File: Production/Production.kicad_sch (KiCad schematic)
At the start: 28 parts, among them IC1 MAX3323EEPE+, J1 530480510, J2 530480410, J3 USB4085-GF-A_REVB, U1 BD33FC0FP-E2, U2 ADR02AUJZ-REEL7, U3 ATSAMD21G18A-AUT, Y1 32.768, 12.5pF

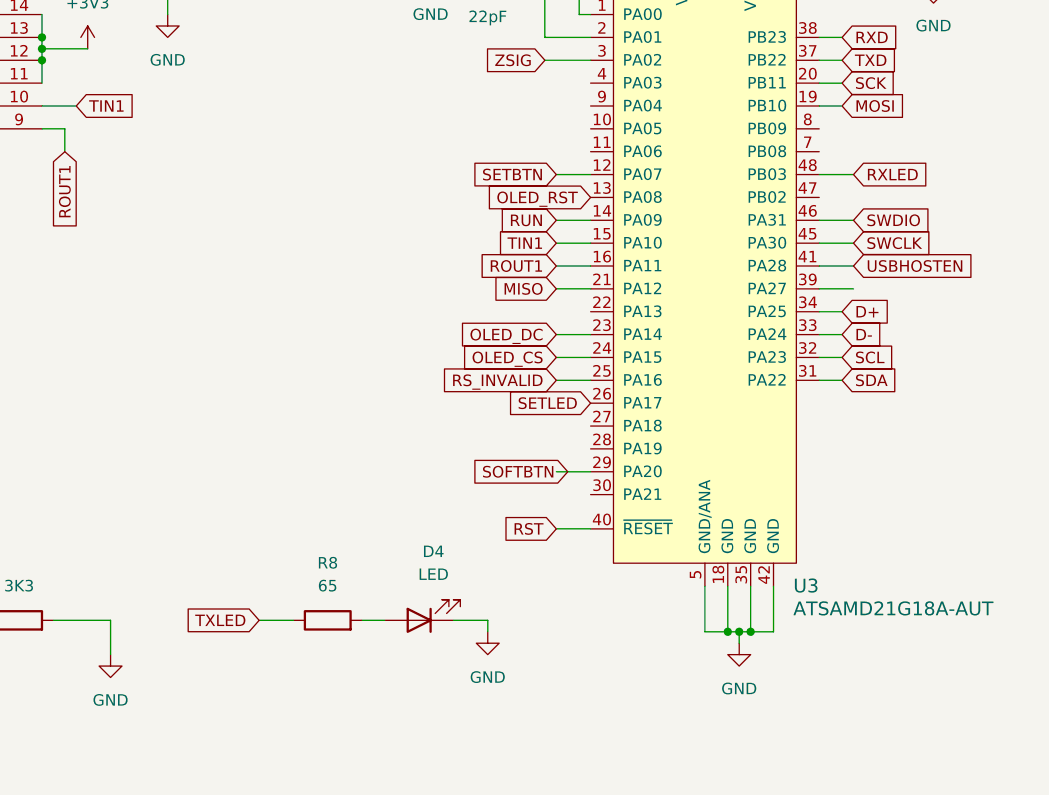
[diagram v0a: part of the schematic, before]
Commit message: I layout
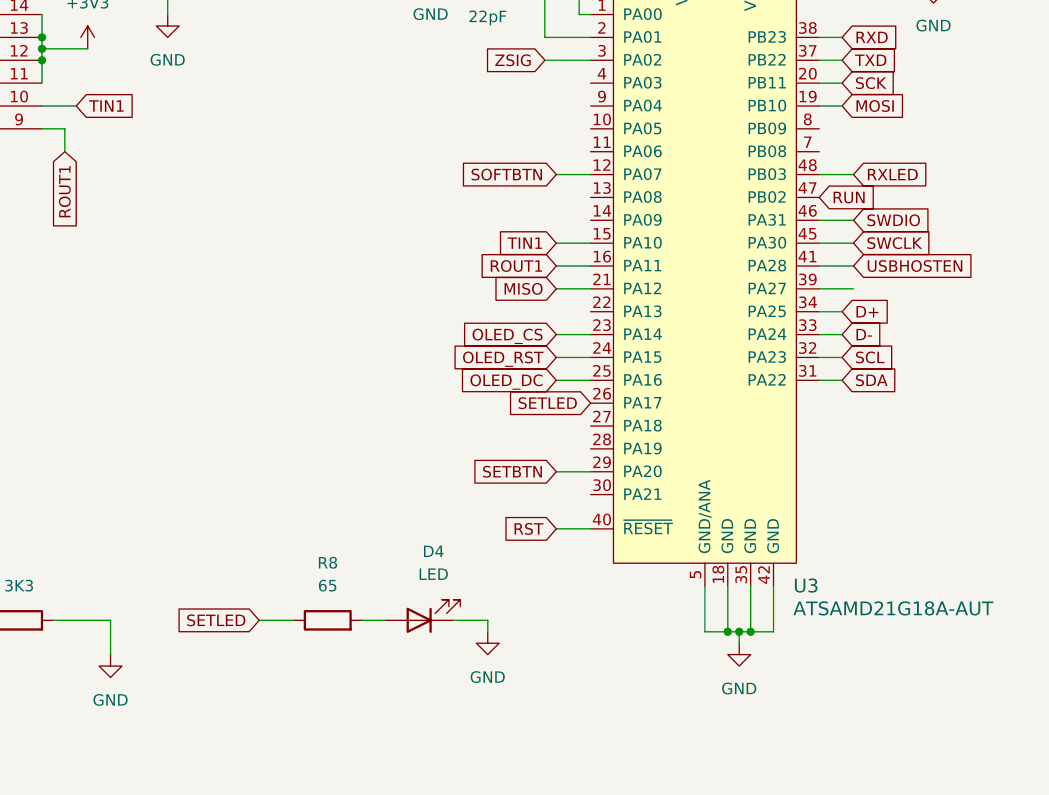
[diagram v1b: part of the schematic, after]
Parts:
- C1, C13, C2, C3, C4, C5, C6, C7, C8: footprint Capacitor_SMD:C_0805_2012Metric -> Capacitor_SMD:C_0504_1310Metric
- J2: footprint Connector_Molex:Molex_PicoBlade_53048-0410_1x04_P1.25mm_Horizontal -> Connector_Molex_2:Molex_PicoBlade_53048-0410_1x04_P1.25mm_Horizontal
- R1, R2, R3, R5, R8: footprint Resistor_SMD:R_0805_2012Metric -> Resistor_SMD:R_0603_1608Metric
- U2: footprint Package_TO_SOT_SMD:TSOT-23-5_HandSoldering -> Package_TO_SOT_SMD:TSOT-23-5
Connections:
- net RS_INVALID is gone; now on net OLED_DC: U3.25 (PA16)
- net TXLED is gone; now on net SETLED: R8.1
- net OLED_CS: now also U3.23 (PA14); no longer U3.24 (PA15)
- net OLED_DC: no longer U3.23 (PA14)
- net OLED_RST: now also U3.24 (PA15); no longer U3.13 (PA08)
- net RUN: now also U3.47 (PB02); no longer U3.14 (PA09)
- net SETBTN: now also U3.29 (PA20); no longer U3.12 (PA07)
- net SOFTBTN: now also U3.12 (PA07); no longer U3.29 (PA20)
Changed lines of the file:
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@@
 	(wire
 		(pts
-			(xy 227.33 99.06) (xy 231.14 99.06)
-		)
-		(stroke
-			(width 0)
-			(type default)
-		)
-	)
-	(wire
-		(pts
 			(xy 105.41 165.1) (xy 107.95 165.1)
 		)
@@
 		)
 	)
-	(global_label "TXLED"
+	(global_label "MOSI"
 		(shape input)
-		(at 194.31 143.51 180)
+		(at 259.08 86.36 0)
 		(fields_autoplaced yes)
 		(effects
@@
 				(size 1.27 1.27)
 			)
-			(justify right)
+			(justify left)
 		)
 		(property "Intersheetrefs" "${INTERSHEET_REFS}"
-			(at 185.7006 143.51 0)
+			(at 266.6614 86.36 0)
 			(effects
 				(font
 					(size 1.27 1.27)
 				)
-				(justify right)
+				(justify left)
 				(hide yes)
 			)
 		)
 	)
-	(global_label "MOSI"
+	(global_label "ZREF"
 		(shape input)
-		(at 259.08 86.36 0)
+		(at 266.7 22.86 90)
 		(fields_autoplaced yes)
 		(effects
@@
 		)
 		(property "Intersheetrefs" "${INTERSHEET_REFS}"
-			(at 266.6614 86.36 0)
+			(at 266.7 15.1577 90)
 			(effects
 				(font
@@
 		)
 	)
-	(global_label "ZREF"
+	(global_label "TXD"
 		(shape input)
-		(at 266.7 22.86 90)
+		(at 259.08 81.28 0)
 		(fields_autoplaced yes)
 		(effects
@@
 		)
 		(property "Intersheetrefs" "${INTERSHEET_REFS}"
-			(at 266.7 15.1577 90)
+			(at 265.5123 81.28 0)
 			(effects
 				(font
@@
 		)
 	)
-	(global_label "TXD"
+	(global_label "SETLED"
 		(shape input)
-		(at 259.08 81.28 0)
+		(at 194.31 143.51 180)
 		(fields_autoplaced yes)
 		(effects
@@
 				(size 1.27 1.27)
 			)
-			(justify left)
+			(justify right)
 		)
 		(property "Intersheetrefs" "${INTERSHEET_REFS}"
-			(at 265.5123 81.28 0)
+			(at 184.5516 143.51 0)
 			(effects
 				(font
 					(size 1.27 1.27)
 				)
-				(justify left)
+				(justify right)
 				(hide yes)
 			)
@@
 	(global_label "OLED_RST"
 		(shape input)
-		(at 231.14 96.52 180)
+		(at 227.33 114.3 180)
 		(fields_autoplaced yes)
 		(effects
@@
 		)
 		(property "Intersheetrefs" "${INTERSHEET_REFS}"
-			(at 218.9625 96.52 0)
+			(at 215.1525 114.3 0)
 			(effects
 				(font
@@
 	(global_label "SOFTBTN"
 		(shape input)
-		(at 228.6 127 180)
+		(at 227.33 93.98 180)
 		(fields_autoplaced yes)
 		(effects
@@
 		)
 		(property "Intersheetrefs" "${INTERSHEET_REFS}"
-			(at 217.4505 127 0)
+			(at 216.1805 93.98 0)
 			(effects
 				(font
@@
 	(global_label "SETBTN"
 		(shape input)
-		(at 227.33 93.98 180)
+		(at 227.33 127 180)
 		(fields_autoplaced yes)
 		(effects
@@
 		)
 		(property "Intersheetrefs" "${INTERSHEET_REFS}"
-			(at 217.4506 93.98 0)
-			(effects
-				(font
-					(size 1.27 1.27)
-				)
-				(justify right)
-				(hide yes)
-			)
-		)
-	)
-	(global_label "RS_INVALID"
-		(shape input)
-		(at 227.33 116.84 180)
-		(fields_autoplaced yes)
-		(effects
-			(font
-				(size 1.27 1.27)
-			)
-			(justify right)
-		)
-		(property "Intersheetrefs" "${INTERSHEET_REFS}"
-			(at 213.8823 116.84 0)
-			(effects
-				(font
-					(size 1.27 1.27)
-				)
-				(justify right)
-				(hide yes)
-			)
-		)
-	)
-	(global_label "RUN"
-		(shape input)
-		(at 227.33 99.06 180)
-		(fields_autoplaced yes)
-		(effects
-			(font
-				(size 1.27 1.27)
-			)
-			(justify right)
-		)
-		(property "Intersheetrefs" "${INTERSHEET_REFS}"
-			(at 220.4138 99.06 0)
+			(at 217.4506 127 0)
 			(effects
 				(font
@@
 		)
 	)
+	(global_label "RUN"
+		(shape input)
+		(at 256.54 96.52 0)
+		(fields_autoplaced yes)
+		(effects
+			(font
+				(size 1.27 1.27)
+			)
+			(justify left)
+		)
+		(property "Intersheetrefs" "${INTERSHEET_REFS}"
+			(at 263.4562 96.52 0)
+			(effects
+				(font
+					(size 1.27 1.27)
+				)
+				(justify left)
+				(hide yes)
+			)
+		)
+	)
 	(global_label "TIN1"
 		(shape input)
@@
 	(global_label "OLED_DC"
 		(shape input)
-		(at 227.33 111.76 180)
+		(at 227.33 116.84 180)
 		(fields_autoplaced yes)
 		(effects
@@
 		)
 		(property "Intersheetrefs" "${INTERSHEET_REFS}"
-			(at 216.0596 111.76 0)
+			(at 216.0596 116.84 0)
 			(effects
 				(font
@@
 	(global_label "OLED_CS"
 		(shape input)
-		(at 227.33 114.3 180)
+		(at 227.33 111.76 180)
 		(fields_autoplaced yes)
 		(effects
@@
 		)
 		(property "Intersheetrefs" "${INTERSHEET_REFS}"
-			(at 216.1201 114.3 0)
+			(at 216.1201 111.76 0)
 			(effects
 				(font
@@
 			)
 		)
-		(property "Footprint" "Capacitor_SMD:C_0805_2012Metric"
+		(property "Footprint" "Capacitor_SMD:C_0504_1310Metric"
 			(at 270.2052 69.85 0)
 			(effects
@@
 			)
 		)
-		(property "Footprint" "Package_TO_SOT_SMD:TSOT-23-5_HandSoldering"
+		(property "Footprint" "Package_TO_SOT_SMD:TSOT-23-5"
 			(at 199.39 27.94 0)
 			(effects
@@
 			)
 		)
-		(property "Footprint" "Capacitor_SMD:C_0805_2012Metric"
+		(property "Footprint" "Capacitor_SMD:C_0504_1310Metric"
 			(at 108.9152 90.17 0)
 			(effects
@@
 			)
 		)
-		(property "Footprint" "Capacitor_SMD:C_0805_2012Metric"
+		(property "Footprint" "Capacitor_SMD:C_0504_1310Metric"
 			(at 118.4148 38.1 0)
 			(effects
@@
 			)
 		)
-		(property "Footprint" "Resistor_SMD:R_0805_2012Metric"
+		(property "Footprint" "Resistor_SMD:R_0603_1608Metric"
 			(at 104.14 156.718 90)
 			(effects
@@
 			)
 		)
-		(property "Footprint" "Capacitor_SMD:C_0805_2012Metric"
+		(property "Footprint" "Capacitor_SMD:C_0504_1310Metric"
 			(at 174.2948 34.29 0)
 			(effects
@@
 			)
 		)
-		(property "Footprint" "Resistor_SMD:R_0805_2012Metric"
+		(property "Footprint" "Resistor_SMD:R_0603_1608Metric"
 			(at 104.14 154.178 90)
 			(effects
@@
 			)
 		)
-		(property "Footprint" "Resistor_SMD:R_0805_2012Metric"
+		(property "Footprint" "Resistor_SMD:R_0603_1608Metric"
 			(at 201.93 145.288 90)
 			(effects
@@
 			)
 		)
-		(property "Footprint" "Capacitor_SMD:C_0805_2012Metric"
+		(property "Footprint" "Capacitor_SMD:C_0504_1310Metric"
 			(at 121.6152 105.41 0)
 			(effects
@@
 			)
 		)
-		(property "Footprint" "Capacitor_SMD:C_0805_2012Metric"
+		(property "Footprint" "Capacitor_SMD:C_0504_1310Metric"
 			(at 108.9152 77.47 0)
 			(effects
@@
 			)
 		)
-		(property "Footprint" "Resistor_SMD:R_0805_2012Metric"
+		(property "Footprint" "Resistor_SMD:R_0603_1608Metric"
 			(at 151.13 145.288 90)
 			(effects
@@
 			)
 		)
-		(property "Footprint" "Resistor_SMD:R_0805_2012Metric"
+		(property "Footprint" "Resistor_SMD:R_0603_1608Metric"
 			(at 167.64 145.288 90)
 			(effects
@@
 			)
 		)
-		(property "Footprint" "Capacitor_SMD:C_0805_2012Metric"
+		(property "Footprint" "Capacitor_SMD:C_0504_1310Metric"
 			(at 223.52 63.8048 0)
 			(effects
@@
 			)
 		)
-		(property "Footprint" "Capacitor_SMD:C_0805_2012Metric"
+		(property "Footprint" "Capacitor_SMD:C_0504_1310Metric"
 			(at 223.52 68.8848 0)
 			(effects
@@
 			)
 		)
-		(property "Footprint" "Connector_Molex:Molex_PicoBlade_53048-0410_1x04_P1.25mm_Horizontal"
+		(property "Footprint" "Connector_Molex_2:Molex_PicoBlade_53048-0410_1x04_P1.25mm_Horizontal"
 			(at 54.61 81.28 0)
 			(effects
@@
 			)
 		)
-		(property "Footprint" "Capacitor_SMD:C_0805_2012Metric"
+		(property "Footprint" "Capacitor_SMD:C_0504_1310Metric"
 			(at 108.9152 105.41 0)
 			(effects
